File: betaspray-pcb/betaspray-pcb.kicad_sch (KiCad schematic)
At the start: 10 parts, among them J1 Conn_01x03_Pin, J2 Conn_01x03_Pin, J3 Conn_01x03_Pin, J4 Conn_01x03_Pin, J5 Conn_01x03_Pin, J6 Conn_01x03_Pin, J7 Conn_01x03_Pin, J9 Conn_01x03_Pin, U1 ESP32-S3, U2 LM3940IT-3.3

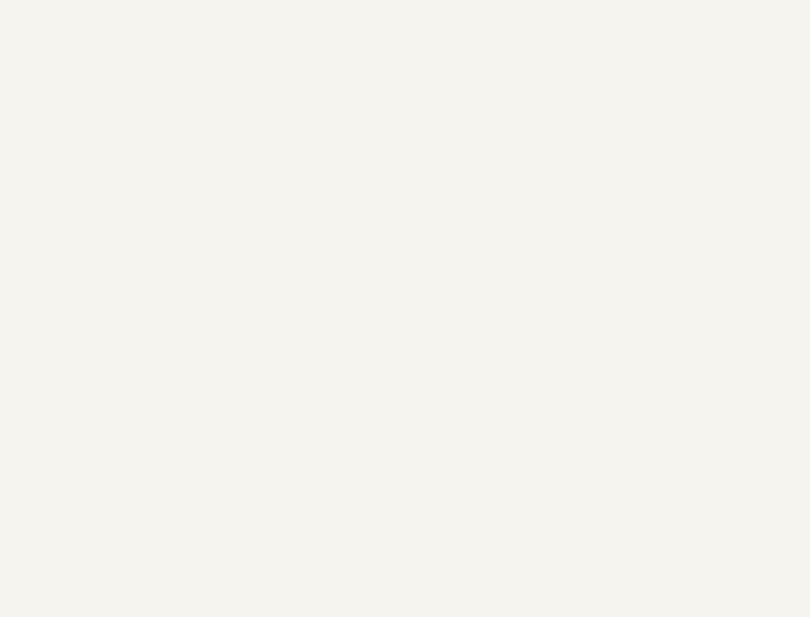
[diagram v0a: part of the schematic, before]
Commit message: Vision subsystem sheet
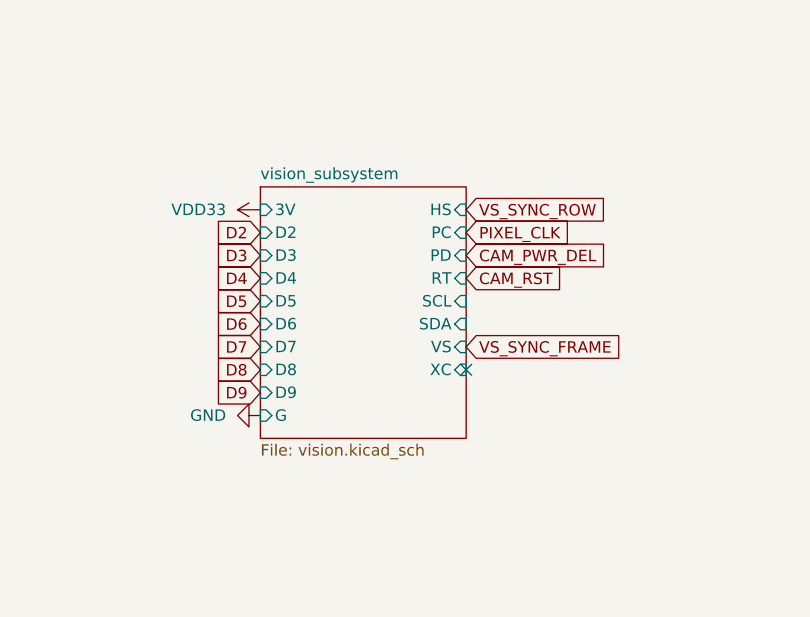
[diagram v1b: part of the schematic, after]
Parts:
- U1: symbol betaspray_MCU_Espressif:ESP32-S3 -> betaspray_Connector:ESP32-S3
- U2: symbol betaspray_LDO:LM3940IT-3.3 -> betaspray_Connector:LM3940IT-3.3
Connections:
- no-connect marks 0 -> 1
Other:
- added sheet vision_subsystem (vision.kicad_sch)
